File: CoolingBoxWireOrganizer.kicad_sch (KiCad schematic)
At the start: 67 parts, among them J1 Conn_02x02_Odd_Even, J10 Conn_01x08_Pin, J11 Conn_02x02_Odd_Even, J12 Conn_02x03_Odd_Even, J13 Conn_01x08_Pin, J14 Conn_01x02, J15 Conn_02x18_Odd_Even, J16 Conn_02x02_Odd_Even, J17 Conn_01x02, J18 DILB16P-223TLF, J19 DILB16P-223TLF, J2 Conn_01x02, J20 Conn_02x03_Odd_Even, J21 Conn_01x02, J22 Conn_01x02, J23 DILB16P-223TLF, J3 Conn_01x08, J4 Conn_01x02, J5 Conn_01x10_Pin, J6 Conn_01x08_Pin, J7 Conn_01x08_Pin, J8 Conn_01x08_Pin, J9 Conn_02x03_Odd_Even, U1 MAX31855KASA, U2 MAX31855KASA, U3 MAX31855KASA, U4 MAX31855KASA

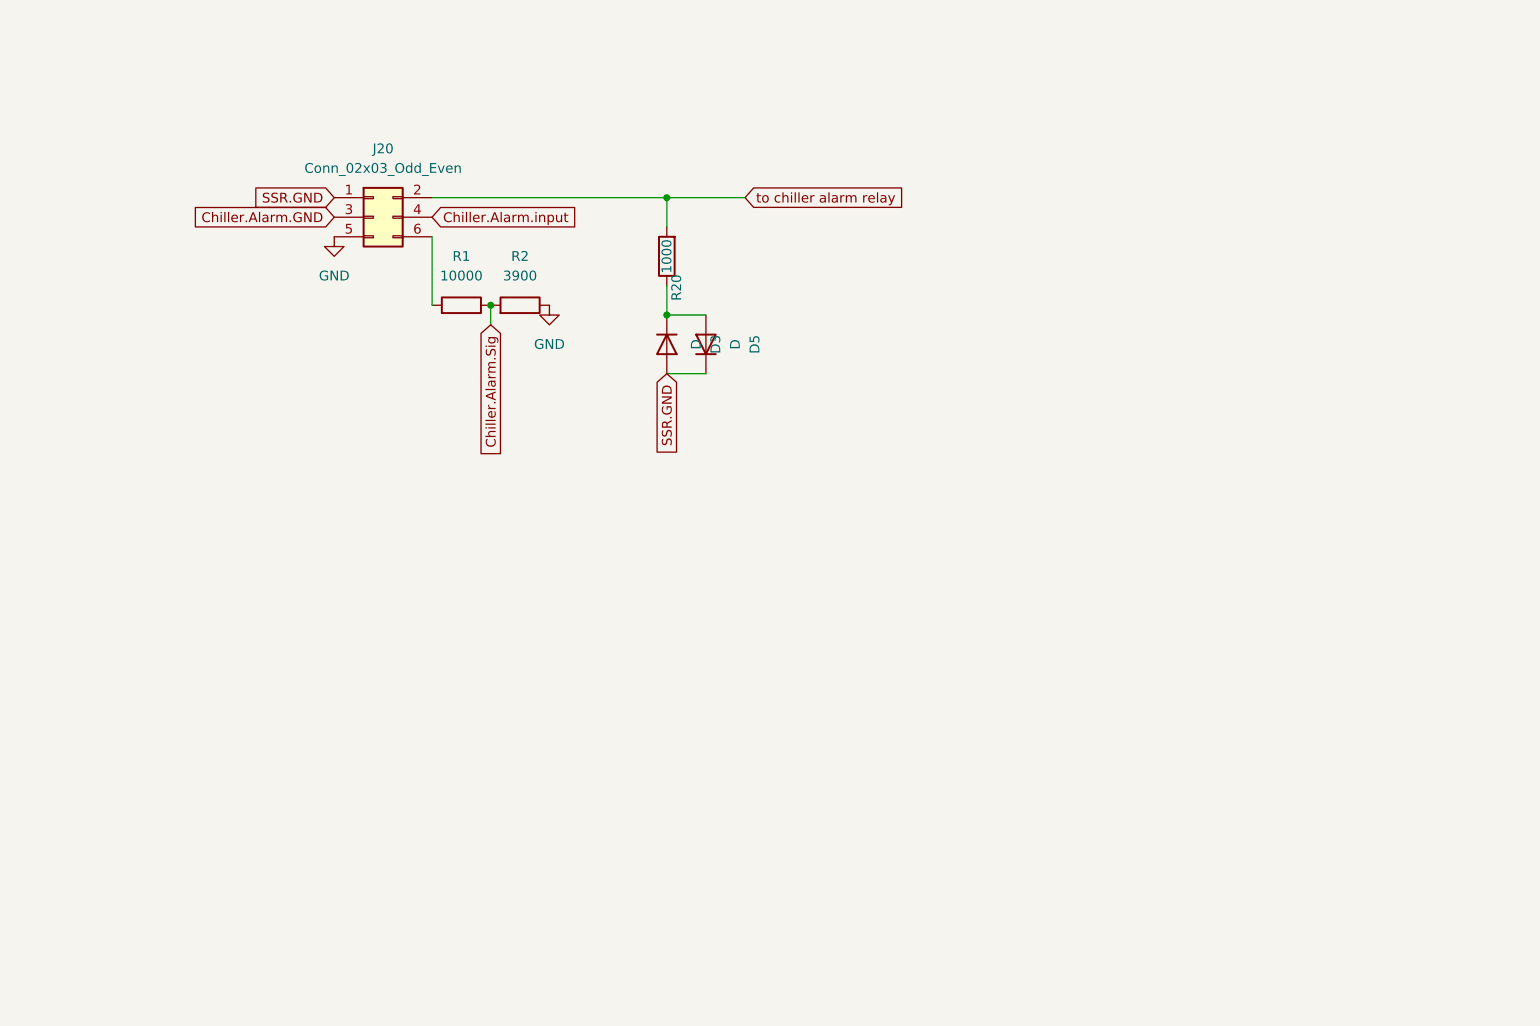
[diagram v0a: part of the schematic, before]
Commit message: trying to change chiller curcuit(on progress)
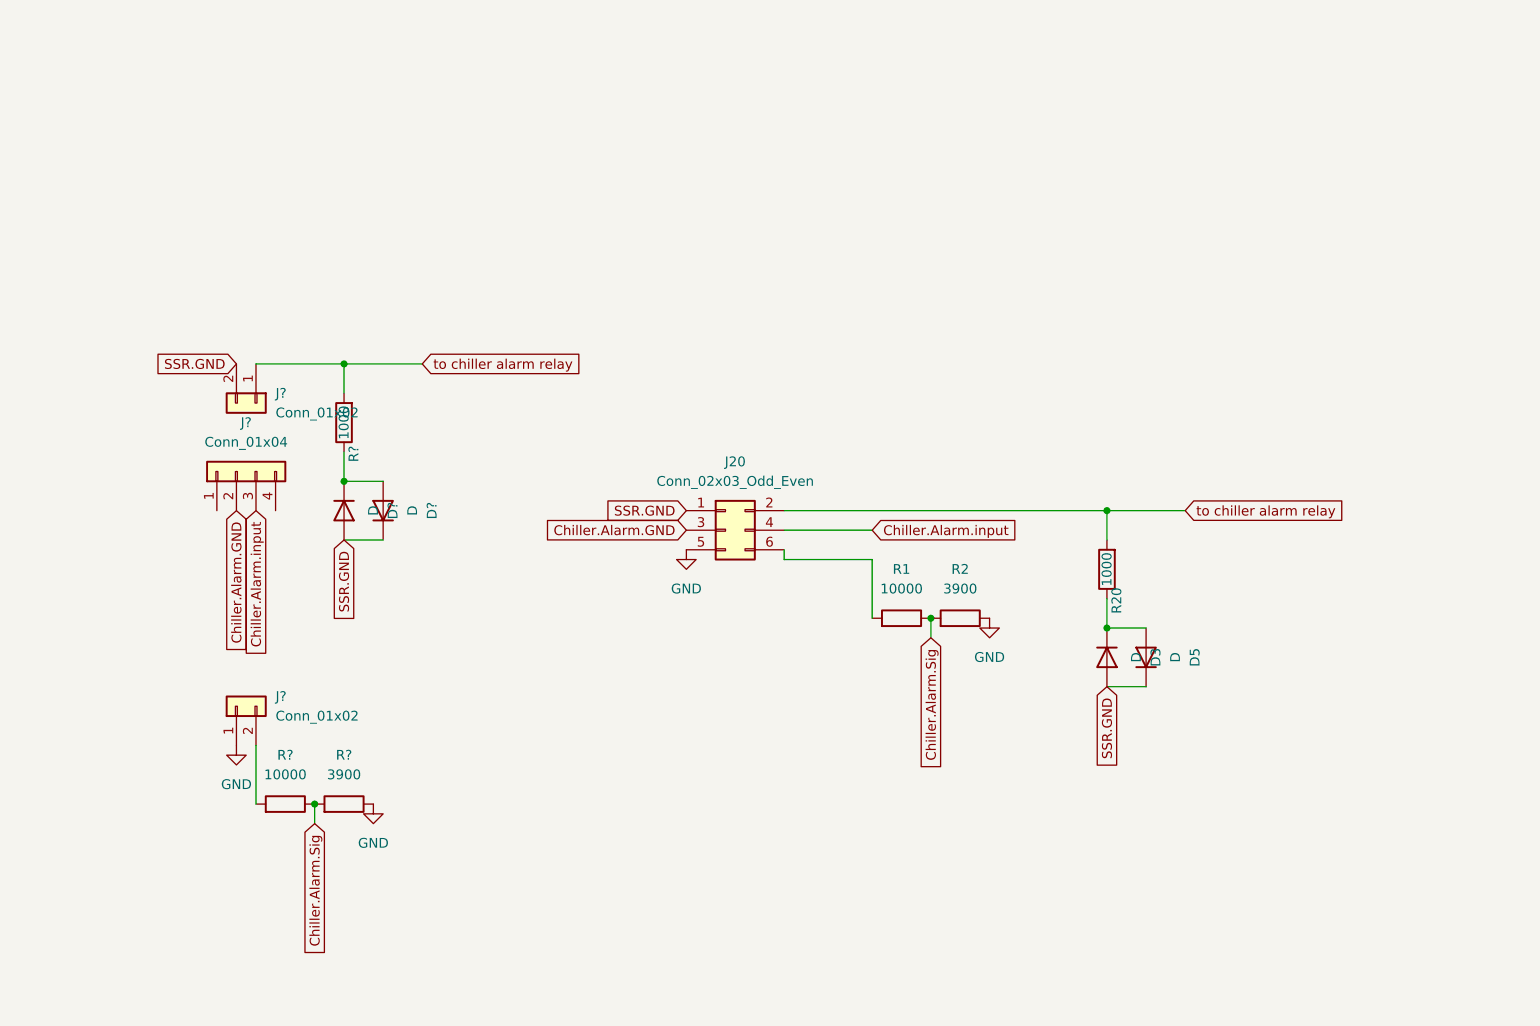
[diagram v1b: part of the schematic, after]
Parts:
- added D? (x2): D, Diode_SMD:D_0603_1608Metric_Pad1.05x0.95mm_HandSolder, symbol Device:D
- added J? (x2): Conn_01x02, symbol Connector_Generic:Conn_01x02
- added J?: Conn_01x04, symbol Connector_Generic:Conn_01x04
- added R?: 1000, Resistor_SMD:R_0603_1608Metric_Pad0.98x0.95mm_HandSolder, symbol Device:R
- added R?: 10000, Resistor_SMD:R_0603_1608Metric_Pad0.98x0.95mm_HandSolder, symbol Device:R
- added R?: 3900, Resistor_SMD:R_0603_1608Metric_Pad0.98x0.95mm_HandSolder, symbol Device:R
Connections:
- net Chiller.Alarm.GND: now also J?.2 (Pin_2)
- net Chiller.Alarm.Sig: now also R?.1, R?.2
- net Chiller.Alarm.input: now also J?.3 (Pin_3)
- net GND: now also J?.1 (Pin_1), R?.1
- net SSR.GND: now also D?.1 (K), D?.2 (A), J?.2 (Pin_2)
- net to chiller alarm relay: now also J?.1 (Pin_1), R?.2
- new net: D?.1 (K), D?.2 (A), R?.1
- new net: J?.2 (Pin_2), R?.2
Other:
- moved on the sheet: D3, D5, J20, R1, R2, R20
